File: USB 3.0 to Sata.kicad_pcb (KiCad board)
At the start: 4 copper layers, 27.8 x 43.5 mm, 38 parts, among them U1 VL716-Q4, U4 XUTS-2205-0429, U5 W25Q16BVSSIG, Y1 25Mhz Crystal

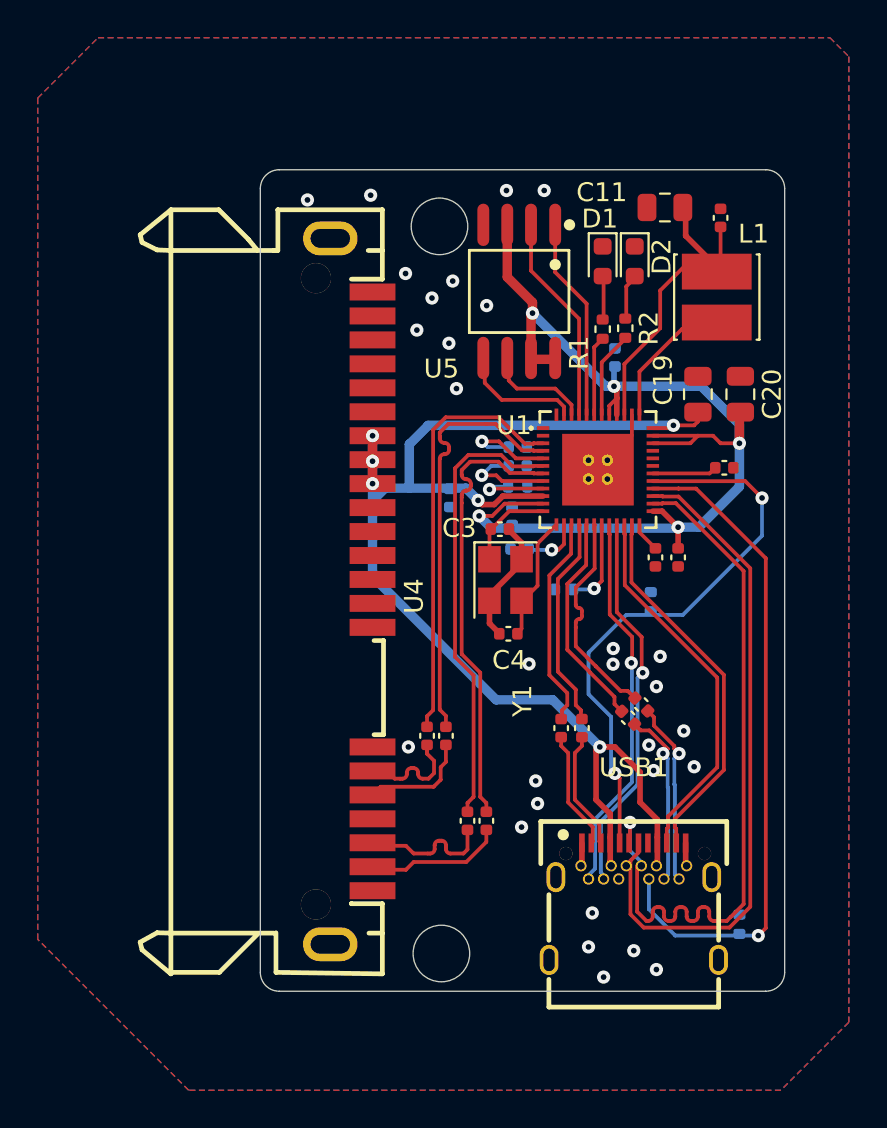
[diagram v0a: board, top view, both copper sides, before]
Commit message: Add files via upload
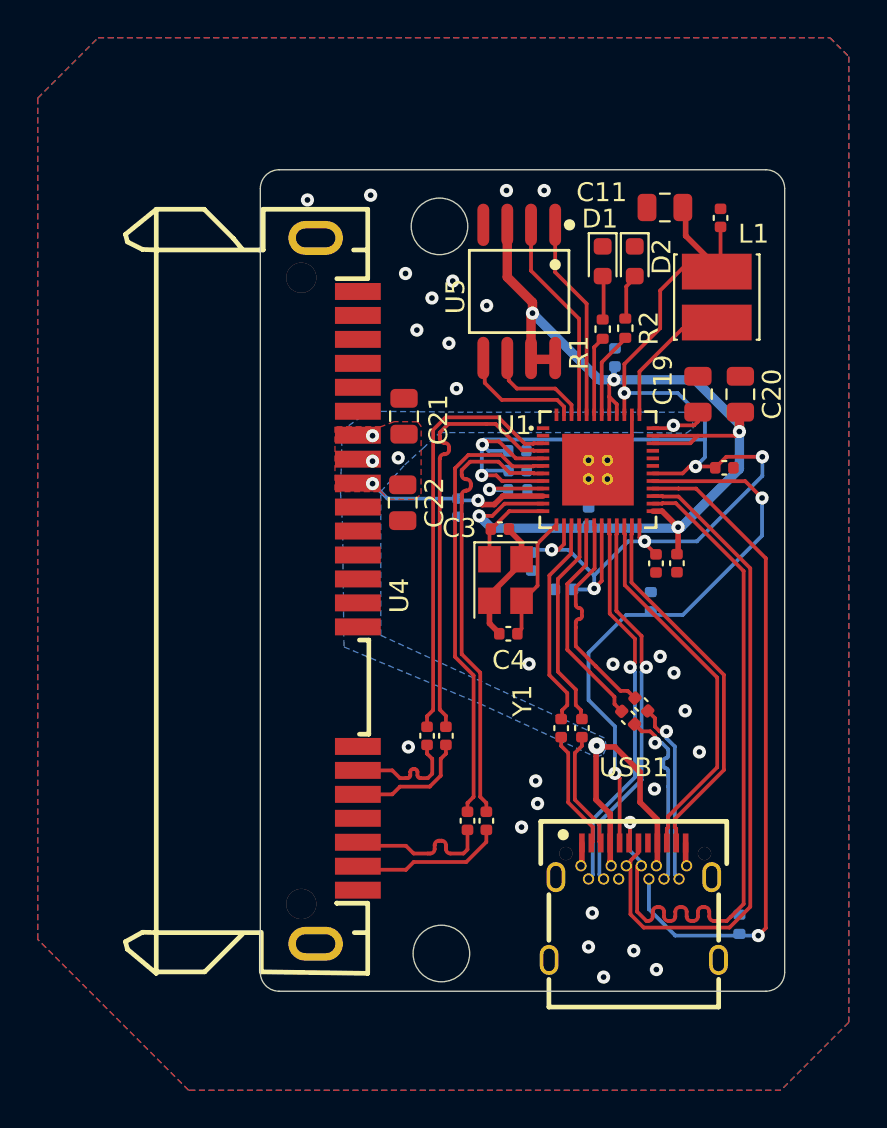
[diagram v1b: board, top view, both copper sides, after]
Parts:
- removed C23, C24: 100nF, Capacitor_SMD:C_0402_1005Metric
- added C21: 22uF, Capacitor_SMD:C_0805_2012Metric, F.Cu at (47.6, 60.1)
- added C22: 22uF, Capacitor_SMD:C_0805_2012Metric, F.Cu at (47.6, 64.7)
- added C29: 100nF, Capacitor_SMD:C_0402_1005Metric, B.Cu at (53.6, 61.9)
- added C30: 100nF, Capacitor_SMD:C_0402_1005Metric, B.Cu at (53.6, 62.9)
- moved C1 4.06 mm to (57.4, 65.4)
- moved C5 0.93 mm to (54.4, 67.8), turned to 90 degrees
- moved U4 0.78 mm to (44.1, 69.3)
- moved C2 0.67 mm to (50.5, 64.9)
- moved C26 0.32 mm to (61.0, 67.9)
- moved C18 0.31 mm to (62.1, 67.9)
- moved R3 0.18 mm to (53.6, 64.0)
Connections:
- C11 pad 1: Net-(U1-DCVCC12) -> U3TXVDD12
- C16 pad 1: Net-(U1-DCVCC12) -> U3TXVDD12
- C17 pad 1: Net-(U1-VDD12I) -> U3TXVDD12
- C25 pad 2: USB3TXVDD12 -> U3TXVDD12
- C26 pad 2: USB3RXVDD12 -> U3TXVDD12
- C5 pad 2: Net-(U1-OSCVDD12) -> U3TXVDD12
- L1 pad 1: Net-(U1-DCVCC12) -> U3TXVDD12
- U1 pad 14: Net-(U1-OSCVDD12) -> U3TXVDD12
- U1 pad 19: USB3TXVDD12 -> U3TXVDD12
- U1 pad 24: USB3RXVDD12 -> U3TXVDD12
- U1 pad 30: Net-(U1-VDD12I) -> U3TXVDD12
- U1 pad 39: Net-(U1-DCVCC12) -> U3TXVDD12
- U1 pad 5: SARXVDD12 -> U3TXVDD12
- U1 pad 8: SATXVDD12 -> U3TXVDD12
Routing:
- net U3TXVDD12: track 0.00 -> 79.8 mm, vias 0 -> 8
- net VBUS: track 69.9 -> 27.4 mm, vias 6 -> 7
- net Net-(U1-DCVCC12): track 16.9 -> 0.00 mm
- net SARXVDD12: track 5.26 -> 0.00 mm, vias 1 -> 0
- net SATXVDD12: track 5.01 -> 0.00 mm, vias 1 -> 0
- net USB3TXVDD12: track 4.70 -> 0.00 mm, vias 1 -> 0
- net Net-(U1-VDD12I): track 3.43 -> 0.00 mm
- net Net-(U1-OSCVDD12): track 3.05 -> 0.00 mm, vias 1 -> 0
- net USB3RXVDD12: track 1.61 -> 0.00 mm
- net +3.3V: track 59.2 -> 58.5 mm
- net /SATA_RXN: track 5.91 -> 6.55 mm
- net RX1+: track 20.1 -> 20.6 mm
- net GND: vias 29 -> 27
- added copper zone on B.Cu, net VBUS
- added copper zone on F.Cu, net VBUS
